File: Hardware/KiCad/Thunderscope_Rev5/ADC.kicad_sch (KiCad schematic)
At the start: 31 parts, among them U6 HMCAD1520

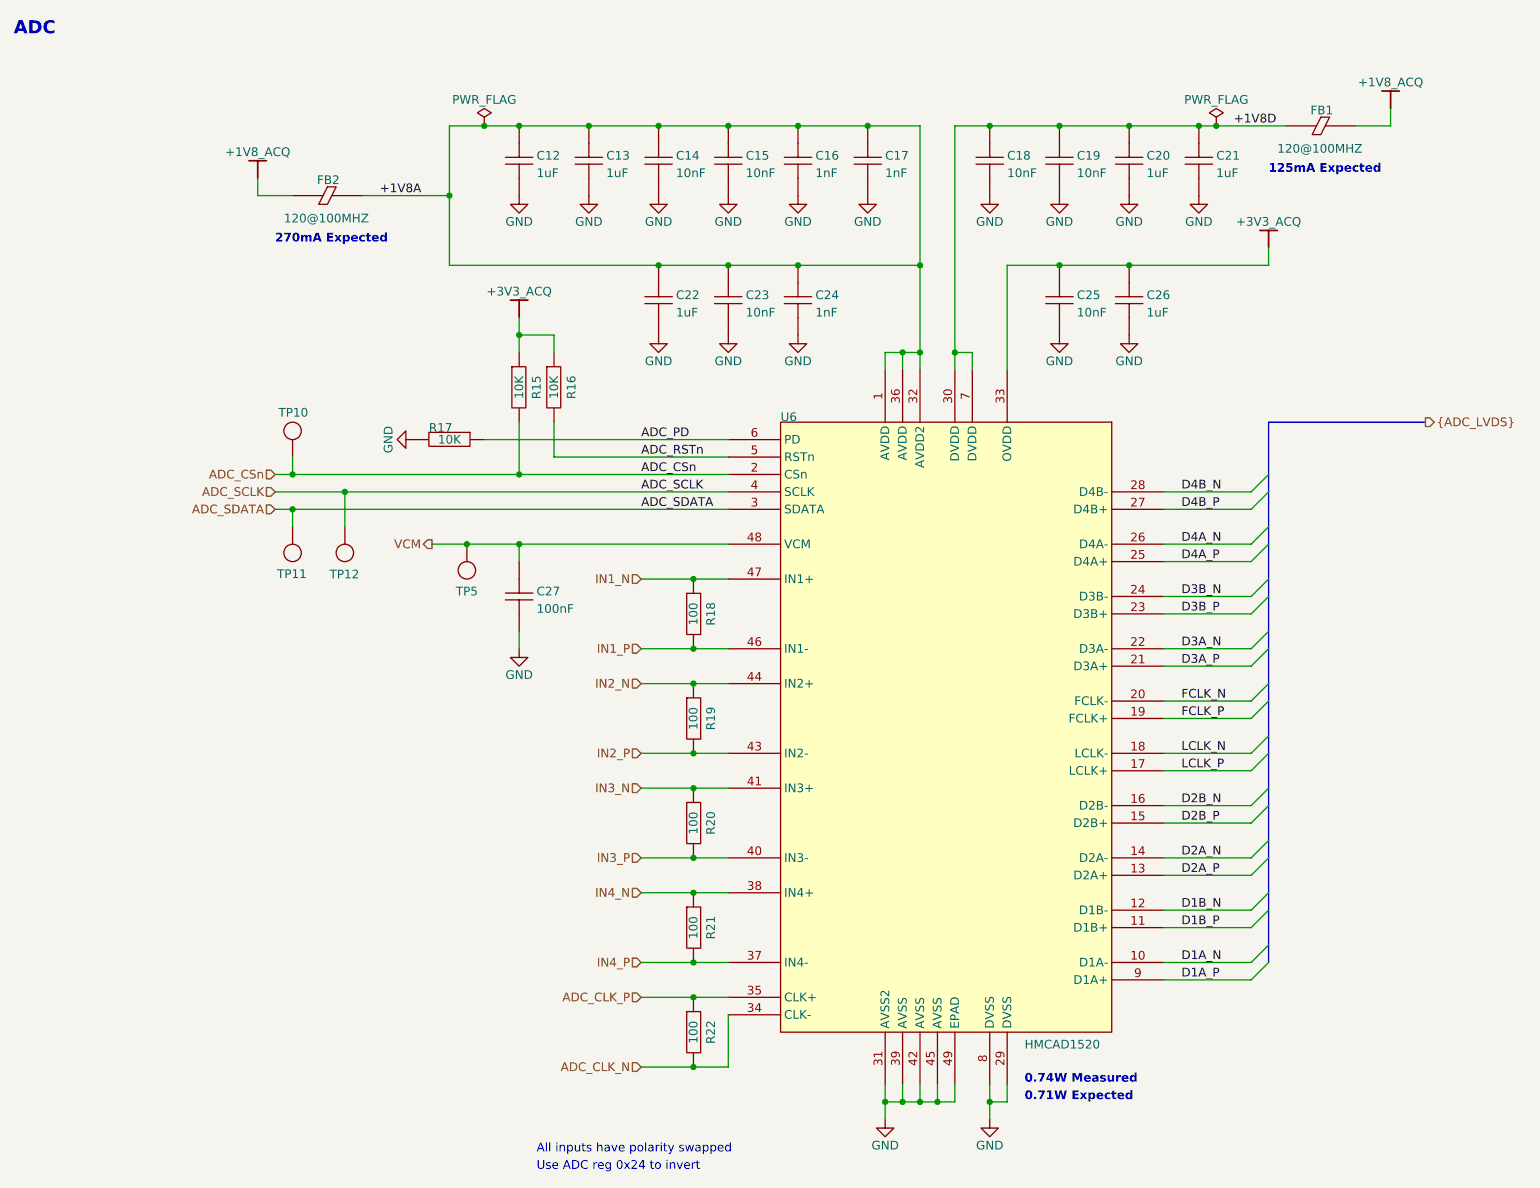
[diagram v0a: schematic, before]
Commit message: Schematic cleanup and RGB status LED
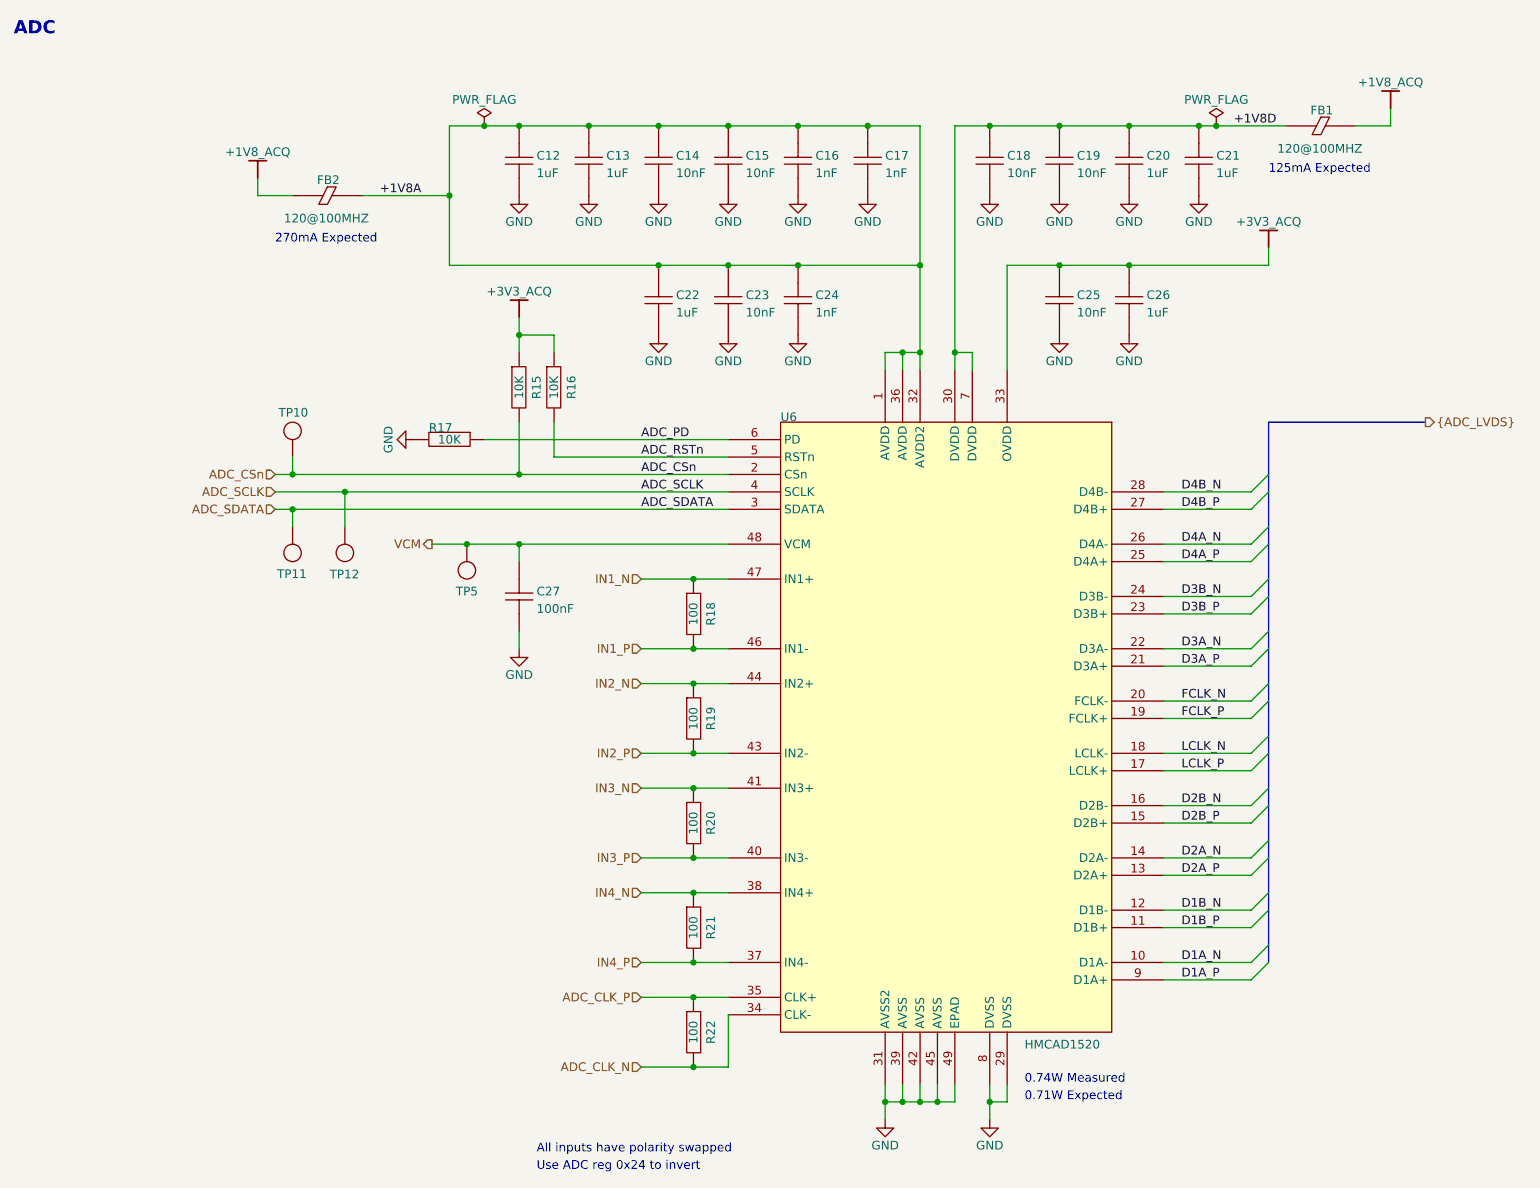
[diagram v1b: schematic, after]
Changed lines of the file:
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@@
 			(font
 				(size 1.27 1.27)
-				(thickness 0.254)
-				(bold yes)
+				(thickness 0.1588)
 			)
 			(justify left)
@@
 			(font
 				(size 1.27 1.27)
-				(thickness 0.254)
-				(bold yes)
+				(thickness 0.1588)
 			)
 			(justify left)
@@
 			(font
 				(size 1.27 1.27)
-				(thickness 0.254)
-				(bold yes)
+				(thickness 0.1588)
 			)
 			(justify left bottom)
@@
 			(font
 				(size 1.27 1.27)
-				(thickness 0.254)
-				(bold yes)
+				(thickness 0.1588)
 			)
 			(justify left bottom)
